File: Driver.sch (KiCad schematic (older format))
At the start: 31 parts, among them J13 CONN_01X10, J14 CONN_01X10, J15 CONN_01X01, J16 CONN_01X01, J17 CONN_01X01, J18 CONN_01X01, Q2 PSMN1R0-40YLD, Q4 PSMN1R0-40YLD, Q5 PSMN1R0-40YLD, Q7 PSMN1R0-40YLD, U4 A4957, U5 ACS722

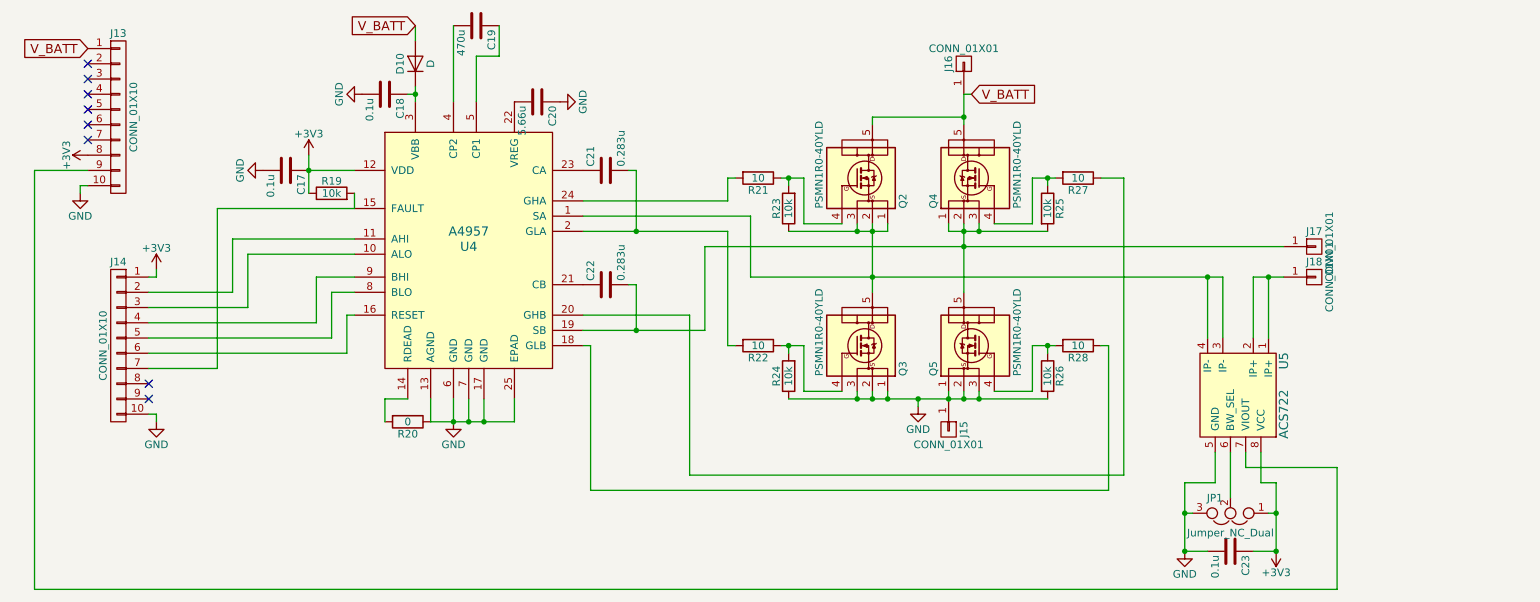
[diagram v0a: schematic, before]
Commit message: FETがパラになったｗｗｗ
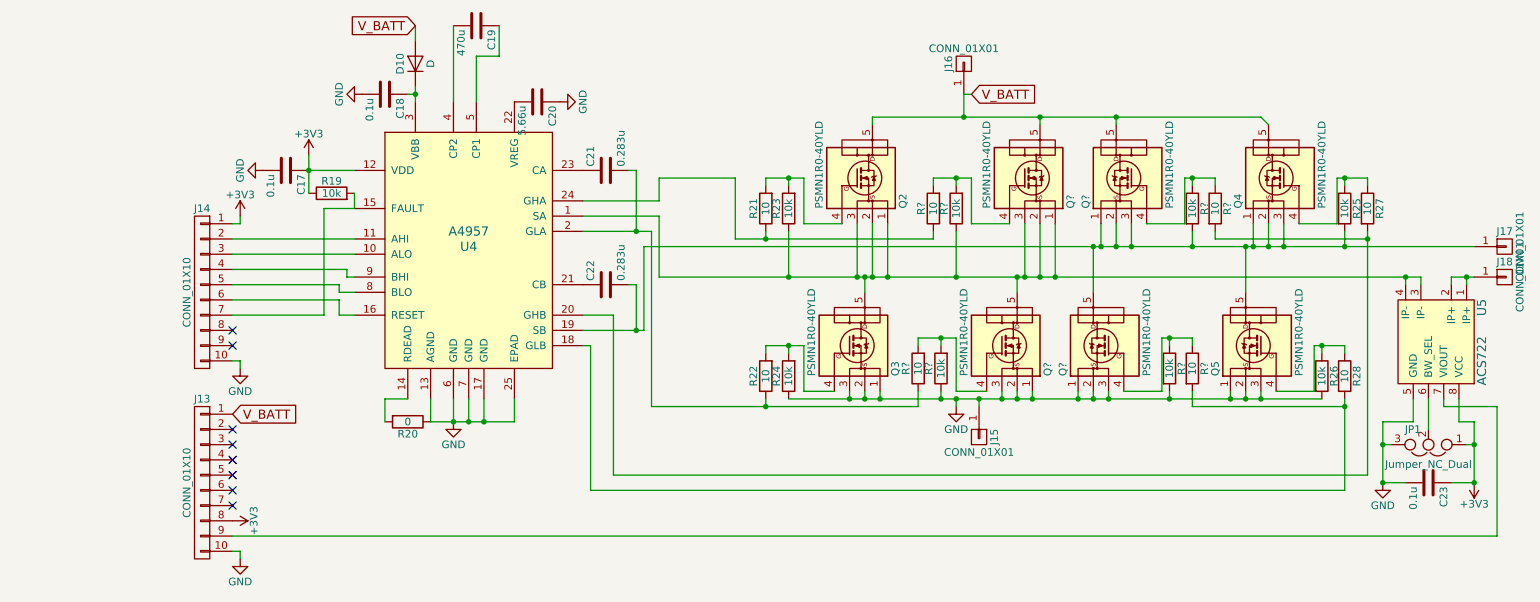
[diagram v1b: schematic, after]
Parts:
- added Q? (x4): PSMN1R0-40YLD, SMD_Packages:LFPAK56_SO8_SOT1023, symbol PSMN1R0-40YLD
- added R? (x4): 10, Resistors_SMD:R_0603, symbol R
- added R? (x4): 10k, Resistors_SMD:R_0603, symbol R
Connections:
- net GND: now also Q?.1 (S), Q?.1 (S), Q?.2 (S), Q?.2 (S), Q?.3 (S), Q?.3 (S), R?.1, R?.2
- net V_BATT: now also Q?.5 (D), Q?.5 (D)
- net at Q2.1 (S), Q2.2 (S), Q2.3 (S)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: now also Q?.1 (S), Q?.2 (S), Q?.3 (S), Q?.5 (D), R?.1
- net at Q2.4 (G), R23.2: now also R21.2; no longer R21.1
- net at Q7.4 (G), R34.2: now also R32.2; no longer R32.1
- net at C29.2, J17.1 (P1), Q4.1 (S)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: now also Q?.1 (S), Q?.2 (S), Q?.3 (S), Q?.5 (D), R?.2
- net at Q4.4 (G), R25.1: now also R27.1; no longer R27.2
- net at Q5.4 (G), R26.1: now also R28.1; no longer R28.2
- net at U4.18 (GLB): now also R28.2, R?.2; no longer R28.1
- net at U4.20 (GHB): now also R27.2, R?.2; no longer R27.1
- net at U4.24 (GHA): now also R21.1, R?.1; no longer R21.2
- net at C21.2, U4.2 (GLA): now also R32.1, R?.1; no longer R32.2
- new net: Q?.4 (G), R?.1, R?.1 (x2)
- new net: Q?.4 (G), R?.2, R?.2 (x2)
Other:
- moved on the sheet: C23, J13, J14, J15, J17, J18, JP1, Q3, Q4, Q5, R21, R22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
